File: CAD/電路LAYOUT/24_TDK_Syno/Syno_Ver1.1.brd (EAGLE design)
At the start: 55.9 x 65.7 mm, 13 parts, among them IC1 REG1117

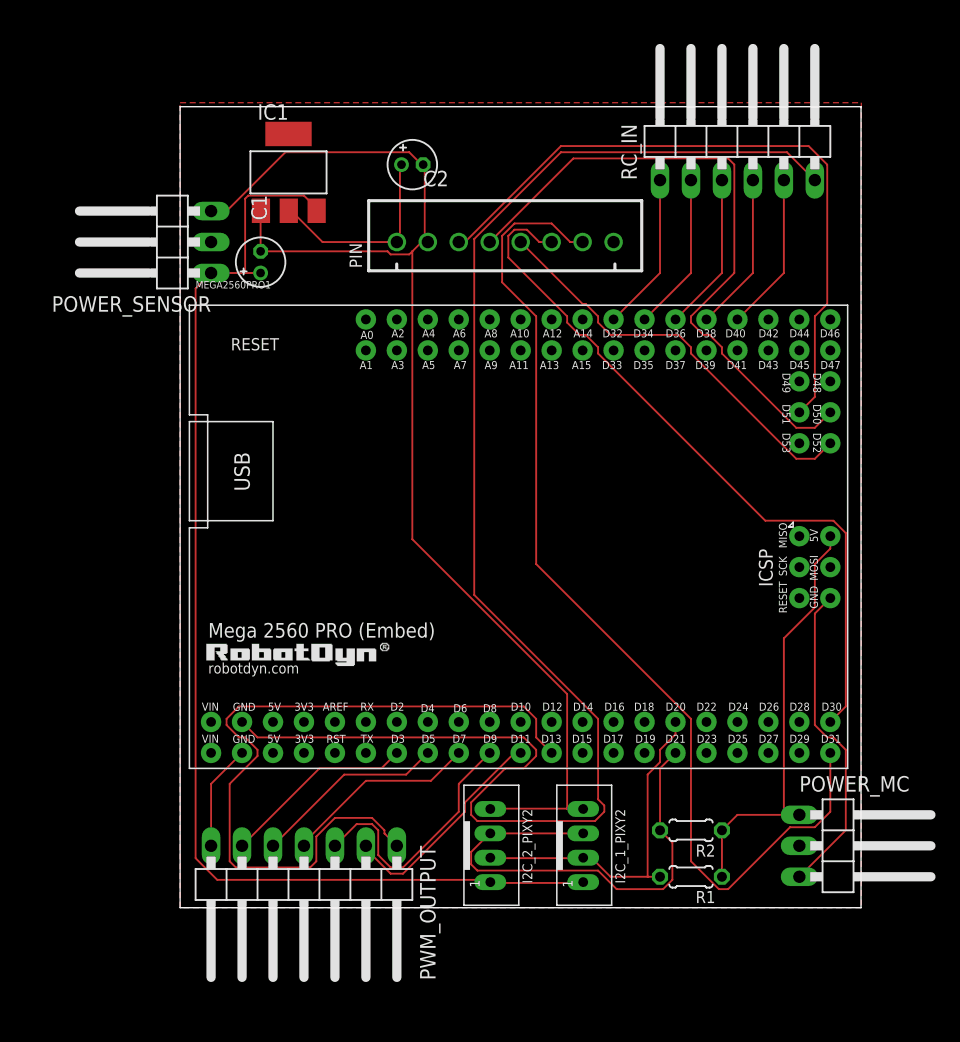
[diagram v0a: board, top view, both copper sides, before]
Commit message: daily update
整理檔案與更新電路Layout(1.0~1.2)
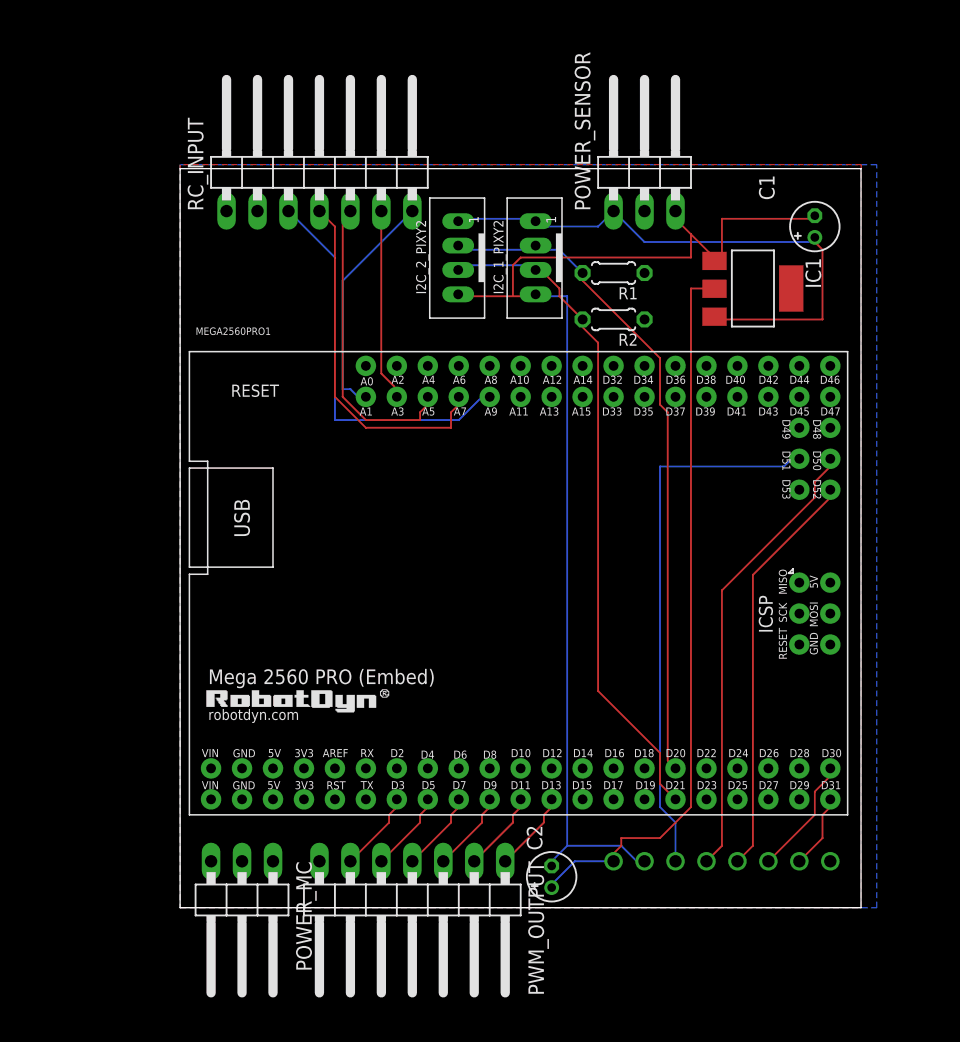
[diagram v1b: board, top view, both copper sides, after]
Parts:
- removed RC_IN: (no value), pinhead:1X06/90
- added RC_INPUT: (no value), pinhead:1X07/90
- moved C2 59.5 mm to (30.5, 2.54), turned to 90 degrees
- moved PIN 53.8 mm to (44.5, 3.81), flipped to the bottom, turned to 180 degrees
- moved R1 49.9 mm to (35.6, 52.1)
- moved POWER_MC 49.8 mm to (5.08, 0.00), turned to 180 degrees
- moved I2C_1_PIXY2 48.4 mm to (29.2, 53.3), turned to 90 degrees
- moved I2C_2_PIXY2 48.3 mm to (22.9, 53.3), turned to 90 degrees
- moved C1 45.6 mm to (52.1, 55.9)
- moved R2 42.4 mm to (35.6, 48.3)
- moved POWER_SENSOR 39.9 mm to (38.1, 61.0), turned to 0 degrees
- moved IC1 39.3 mm to (47.0, 50.8), turned to 270 degrees
- moved PWM_OUTPUT 8.98 mm to (19.1, 0.00)
- moved MEGA2560PRO1 3.81 mm to (35.6, 27.9)
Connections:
- removed net N$18: MEGA2560PRO1.D40, RC_IN.5
- removed net N$19: MEGA2560PRO1.GND@2, RC_IN.6
- net 5V: now also MEGA2560PRO1.5V@1, MEGA2560PRO1.5V@2, RC_INPUT.1
- net GND: now also MEGA2560PRO1.GND@1, MEGA2560PRO1.GND@2, PWM_OUTPUT.7, RC_INPUT.2
- net N$13: now also MEGA2560PRO1.A9, RC_INPUT.3; no longer MEGA2560PRO1.GND@1, PWM_OUTPUT.7
- net N$14: now also MEGA2560PRO1.A7, RC_INPUT.4; no longer MEGA2560PRO1.D32, RC_IN.1
- net N$15: now also MEGA2560PRO1.A5, RC_INPUT.5; no longer MEGA2560PRO1.D34, RC_IN.2
- net N$16: now also MEGA2560PRO1.A3, RC_INPUT.6; no longer MEGA2560PRO1.D36, RC_IN.3
- net N$17: now also MEGA2560PRO1.A1, RC_INPUT.7; no longer MEGA2560PRO1.D38, RC_IN.4
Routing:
- net N$19: track 128.2 -> 0.00 mm
- net N$6: track 85.2 -> 6.13 mm
- net N$7: track 61.4 -> 6.66 mm
- net 5V_S: track 98.0 -> 47.7 mm
- net N$5: track 59.6 -> 9.72 mm
- net N$2: track 16.5 -> 59.5 mm
- net 5V: track 35.1 -> 0.00 mm
- net SDA: track 28.2 -> 55.5 mm
- net GND: track 26.3 -> 0.00 mm
- net N$13: track 8.67 -> 32.2 mm
- net N$3: track 53.4 -> 37.2 mm
- net N$14: track 13.0 -> 29.1 mm
- net SCL: track 39.9 -> 55.7 mm
- net N$9: track 21.3 -> 6.66 mm
- net N$18: track 13.0 -> 0.00 mm
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- added copper zone on layer 1, net 5V
- added copper zone on layer 16, net GND
- removed copper zone on layer 1, net DONT_TIUCH
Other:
- board size 55.9 x 65.7 mm -> 55.9 x 60.6 mm
